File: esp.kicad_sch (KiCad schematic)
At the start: 29 parts, among them J1 Barrel_Jack, J2 8P8C_Shielded, J21 8P8C_Shielded, J3 Barrel_Jack, J38 8P8C_Shielded, J4 Barrel_Jack, J5 Barrel_Jack, J7 Barrel_Jack_MountingPin, K1 RT314A24, P1 Conn_WallPlug_Earth, U1 ESP32-S2-WROVER, U14 PCF8574ATS, U16 L298N, U17 PCA9685PW, U18 NID30S48-24, U2 TCA9548ARGER, U3 TCA9548ARGER, U4 BME280, U6 PCF8574ATS, U7 OKI-78SR-12_1.0-W36H-C, U8 OKI-78SR-5_1.5-W36-C, U9 OKI-78SR-3.3_1.5-W36H-C

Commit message: main sheet barrel connector
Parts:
- removed U14, U6: PCF8574ATS, Package_SO:SSOP-20_4.4x6.5mm_P0.65mm, symbol Interface_Expansion:PCF8574ATS
- removed U17: PCA9685PW, Package_SO:TSSOP-28_4.4x9.7mm_P0.65mm, symbol Driver_LED:PCA9685PW
- added C2, C3, C4, C5: 220uF, symbol Device:C_Polarized_Small_US
- added D10, D11, D12, D13, D14, D15, D16, D17, D18, D19, D20, D21, D22, D23, D24, D25, D26, D27, D28, D29, D30, D31, D32, D33, D34, D35, D36, D37, D38, D39, D40, D9: 1N4001, Diode_THT:D_DO-41_SOD81_P10.16mm_Horizontal, symbol Diode:1N4001
- added F10, F11, F12, F13, F14, F37, F38, F9: Fuse, symbol Device:Fuse
- added F39, F40, F41, F42, F43, F45, F46, F8: U6_P2, symbol Device:Polyfuse_Small
- added J11, J12, J13, J14, J27, J39, J40, J42, J43, J44, J46, J47: Barrel_Jack, symbol Connector:Barrel_Jack
- added Q10, Q11, Q3, Q4, Q5, Q6, Q7, Q8: MOSFET-NCHANNELSMD, Logic_Level_Bidirectional:SOT23-3, symbol Logic_Level_Bidirectional-eagle-import:MOSFET-NCHANNELSMD
- added R10, R11, R12, R13, R14, R15, R16, R17, R18, R20, R21, R23, R24, R7, R8, R9: 10K, Logic_Level_Bidirectional:0603-RES, symbol Logic_Level_Bidirectional-eagle-import:RESISTOR0603-RES
- added U14, U17, U6: L298N, Package_TO_SOT_THT:TO-220-15_P2.54x2.54mm_StaggerOdd_Lead4.58mm_Vertical, symbol Driver_Motor:L298N
- added U15, U20, U5: PCF8574ATS, Package_SO:SSOP-20_4.4x6.5mm_P0.65mm, symbol Interface_Expansion:PCF8574ATS
- added U19: PCA9685PW, Package_SO:TSSOP-28_4.4x9.7mm_P0.65mm, symbol Driver_LED:PCA9685PW
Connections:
- net +12V: now also U16.4 (Vs), C2.1, C3.1, C4.1, C5.1, D11.1 (K), D13.1 (K), D15.1 (K), D17.1 (K), D19.1 (K), D21.1 (K), D23.1 (K), D25.1 (K), D27.1 (K), D29.1 (K), D31.1 (K), D33.1 (K), D35.1 (K), D37.1 (K), D39.1 (K), D9.1 (K), U14.4 (Vs), U17.4 (Vs), U6.4 (Vs); no longer U16.9 (Vss)
- net +3.3V: now also Q10.1 (G), Q11.1 (G), Q3.1 (G), Q4.1 (G), Q5.1 (G), Q6.1 (G), Q7.1 (G), Q8.1 (G), R10.1, R12.1, R16.1, R17.1, R18.1, R23.1, R24.1, R8.1, U5.15 (VSS)
- net GND: now also U16.1 (SENSE_A), C2.2, C3.2, C4.2, C5.2, D10.2 (A), D12.2 (A), D14.2 (A), D16.2 (A), D18.2 (A), D20.2 (A), D22.2 (A), D24.2 (A), D26.2 (A), D28.2 (A), D30.2 (A), D32.2 (A), D34.2 (A), D36.2 (A), D38.2 (A), D40.2 (A), J11.2, J39.2, J40.2, J42.2, J43.2, J44.2, J46.2, J47.2, U14.1 (SENSE_A), U14.8 (GND), U15.6 (A0), U17.1 (SENSE_A), U17.8 (GND), U20.6 (A0), U20.7 (A1), U5.5 (VDD), U5.7 (A1), U5.9 (A2), U6.1 (SENSE_A), U6.8 (GND)
- net at J5.1: now also F12.1
- net at J5.2: now also D23.2 (A), D24.1 (K), U6.2 (OUT1)
- net at U3.1 (SD0): now also U15.4 (SDA)
- net at U3.12 (SD5): now also U5.4 (SDA)
- net at U3.13 (SC5): now also U5.2 (SCL)
- net at U3.19 (SCL): now also U1.20 (IO17)
- net at U3.2 (SC0): now also U15.2 (SCL)
- net at U3.20 (SDA): now also U1.19 (IO16)
- net at U3.3 (SD1): now also U19.27 (SDA)
- net at U3.4 (SC1): now also U19.26 (SCL)
- net at U3.5 (SD2): now also U20.4 (SDA)
- net at U3.6 (SC2): now also U20.2 (SCL)
- net at J4.1: now also F11.1
- net at J4.2: now also D19.2 (A), D20.1 (K), U6.13 (OUT3)
- net at U16.10 (IN3): now also U20.19 (P6)
- net at U16.11 (EnB): now also U19.13 (LED7)
- net at U16.12 (IN4): now also U20.20 (P7)
- net at U16.13 (OUT3): now also D29.2 (A), D30.1 (K), J12.2
- net at U16.14 (OUT4): now also D25.2 (A), D26.1 (K), F13.2
- net at U16.2 (OUT1): now also D37.2 (A), D38.1 (K), J13.2
- net at U16.3 (OUT2): now also D33.2 (A), D34.1 (K), F14.2
- net at U16.5 (IN1): now also U20.16 (P4)
- net at U16.6 (EnA): now also U19.12 (LED6)
- net at U16.7 (IN2): now also U20.17 (P5)
- net at J1.1: now also F9.1
- net at J1.2: now also D11.2 (A), D12.1 (K), U14.13 (OUT3)
- net at J3.1: now also F10.1
- net at J3.2: now also D15.2 (A), D16.1 (K), U14.2 (OUT1)
- new net: F13.1, J12.1
- new net: F46.1, J47.1
- new net: D17.2 (A), D18.1 (K), F11.2, U6.14 (OUT4)
- new net: D13.2 (A), D14.1 (K), F10.2, U14.3 (OUT2)
- new net: F37.1, J14.1
- new net: D31.2 (A), D32.1 (K), J14.2, U17.13 (OUT3)
- new net: F43.1, J44.1
- new net: F42.1, J43.1
- new net: D10.1 (K), D9.2 (A), F9.2, U14.14 (OUT4)
- new net: F8.1, J11.1
- new net: D27.2 (A), D28.1 (K), F37.2, U17.14 (OUT4)
- new net: D39.2 (A), D40.1 (K), J27.2, U17.2 (OUT1)
- new net: F45.1, J46.1
- new net: D21.2 (A), D22.1 (K), F12.2, U6.3 (OUT2)
- new net: F41.1, J42.1
- new net: U17.6 (EnA), U19.10 (LED4)
- new net: U17.11 (EnB), U19.11 (LED5)
- new net: U14.6 (EnA), U19.6 (LED0)
- new net: U14.11 (EnB), U19.7 (LED1)
- new net: U19.8 (LED2), U6.6 (EnA)
- new net: U19.9 (LED3), U6.11 (EnB)
- new net: F39.1, J39.1
- new net: U17.5 (IN1), U20.10 (P0)
- new net: U17.7 (IN2), U20.11 (P1)
- new net: U17.10 (IN3), U20.12 (P2)
- new net: U17.12 (IN4), U20.14 (P3)
- new net: U14.5 (IN1), U15.10 (P0)
- new net: U14.7 (IN2), U15.11 (P1)
- new net: U14.10 (IN3), U15.12 (P2)
- new net: U14.12 (IN4), U15.14 (P3)
- new net: U15.16 (P4), U6.5 (IN1)
- new net: U15.17 (P5), U6.7 (IN2)
- new net: U15.19 (P6), U6.10 (IN3)
- new net: U15.20 (P7), U6.12 (IN4)
- new net: F14.1, J13.1
- new net: F40.1, J40.1
- new net: D35.2 (A), D36.1 (K), F38.2, U17.3 (OUT2)
- new net: F38.1, J27.1
- new net +5V: R11.1, R13.1, R14.1, R15.1, R20.1, R21.1, R7.1, R9.1
- new net HV4: F39.2, F40.2, F41.2, F42.2, F43.2, F45.2, F46.2, F8.2, Q10.3 (D), Q11.3 (D), Q3.3 (D), Q4.3 (D), Q5.3 (D), Q6.3 (D), Q7.3 (D), Q8.3 (D), R11.2, R13.2, R14.2, R15.2, R20.2, R21.2, R7.2, R9.2
- new net LV4: Q10.2 (S), Q11.2 (S), Q3.2 (S), Q4.2 (S), Q5.2 (S), Q6.2 (S), Q7.2 (S), Q8.2 (S), R10.2, R12.2, R16.2, R17.2, R18.2, R23.2, R24.2, R8.2, U5.10 (P0), U5.11 (P1), U5.12 (P2), U5.14 (P3), U5.16 (P4), U5.17 (P5), U5.19 (P6), U5.20 (P7)
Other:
- moved on the sheet: BT1, BT2, F1, F2, F3, F5, J2, J21, J38, J7, K1, P1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

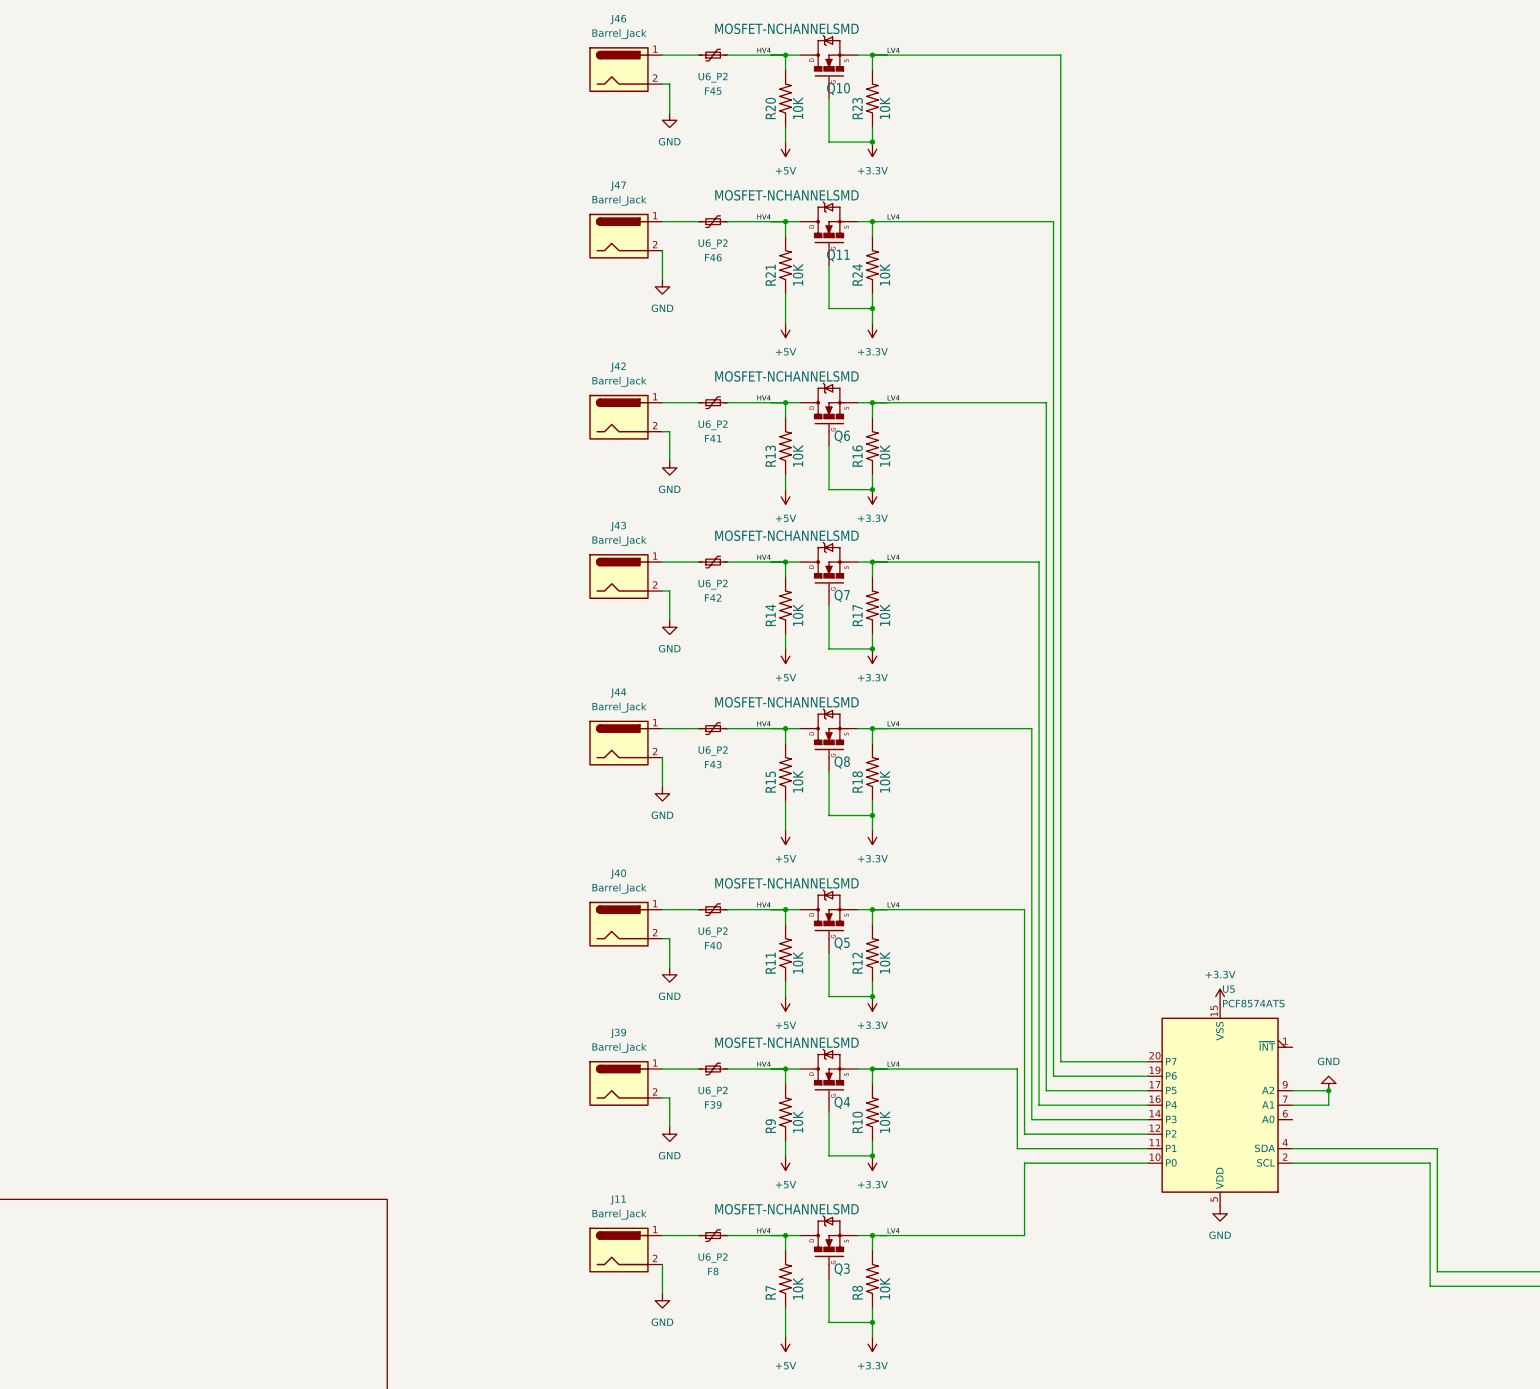
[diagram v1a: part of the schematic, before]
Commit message: add some relay stuff, not complete
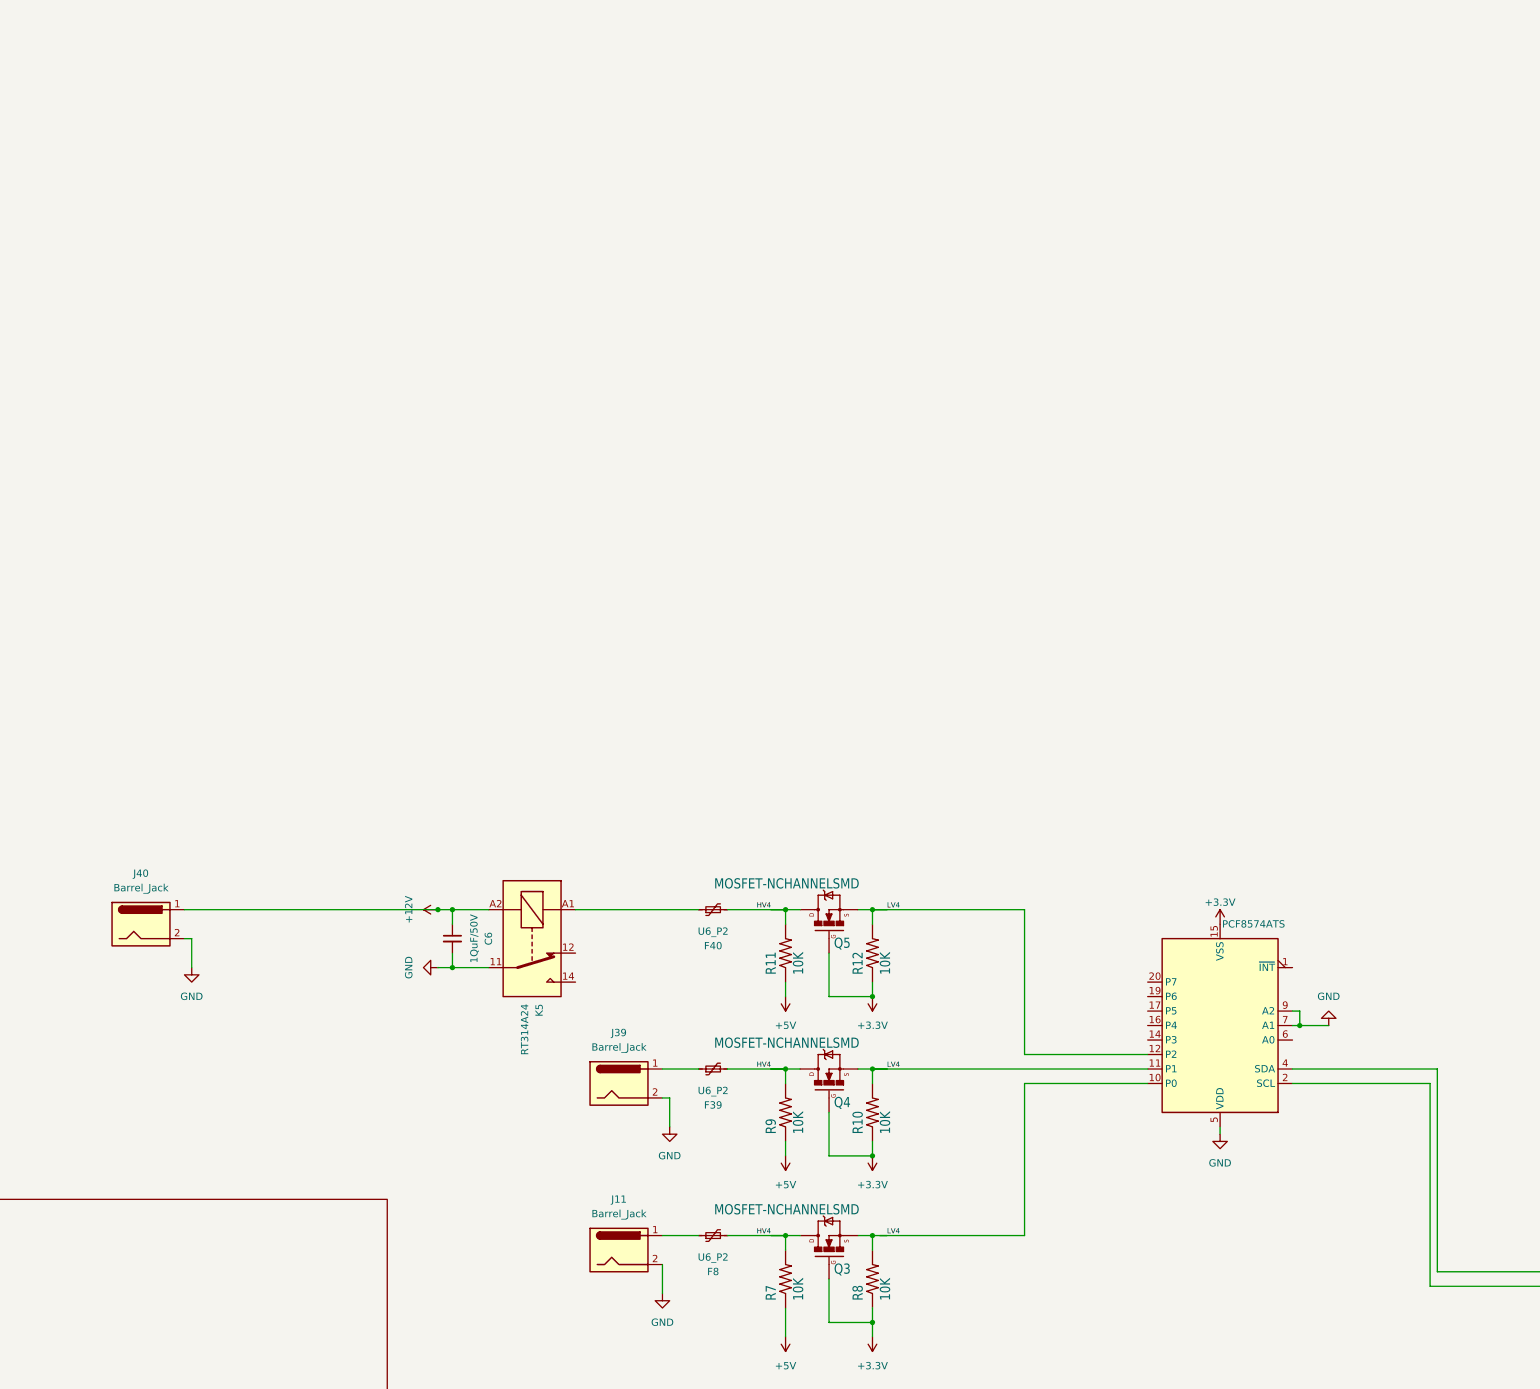
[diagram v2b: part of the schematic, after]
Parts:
- removed F41, F42, F43, F45, F46: U6_P2, symbol Device:Polyfuse_Small
- removed J42, J43, J44, J46, J47: Barrel_Jack, symbol Connector:Barrel_Jack
- removed Q10, Q11, Q6, Q7, Q8: MOSFET-NCHANNELSMD, Logic_Level_Bidirectional:SOT23-3, symbol Logic_Level_Bidirectional-eagle-import:MOSFET-NCHANNELSMD
- removed R13, R14, R15, R16, R17, R18, R20, R21, R23, R24: 10K, Logic_Level_Bidirectional:0603-RES, symbol Logic_Level_Bidirectional-eagle-import:RESISTOR0603-RES
- added C6: 1QuF/50V, symbol Device:C_Small
- added K5: RT314A24, Relay_THT:Relay_SPDT_Schrack-RT1-16A-FormC_RM5mm, symbol Relay:RT314A24
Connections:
- net +12V: now also J40.1, C6.1, K5.A2
- net GND: now also C6.2, K5.11
- net LV4: no longer U5.14 (P3), U5.16 (P4), U5.17 (P5), U5.19 (P6), U5.20 (P7)
- net at F40.1: now also K5.A1; no longer J40.1
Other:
- moved on the sheet: J40
